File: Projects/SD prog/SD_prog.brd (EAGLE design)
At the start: 11 x 24.6 mm, 6 parts

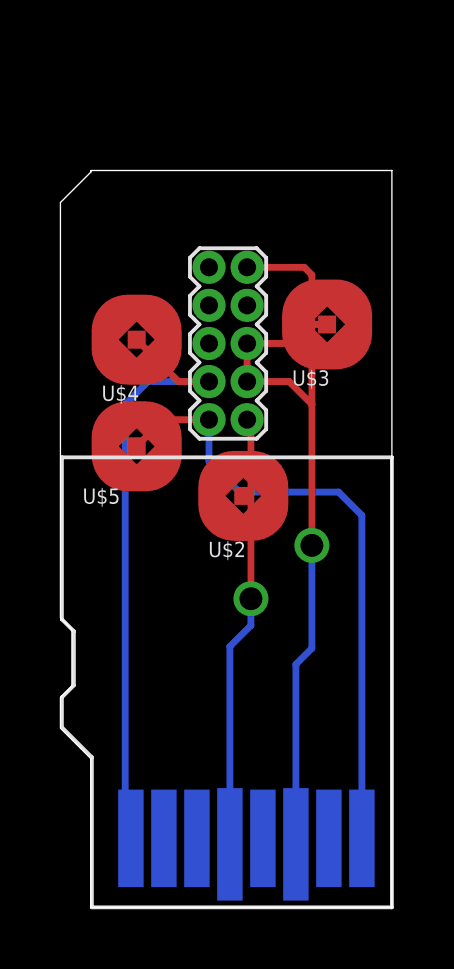
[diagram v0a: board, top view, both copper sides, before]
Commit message: Order @ Boktech
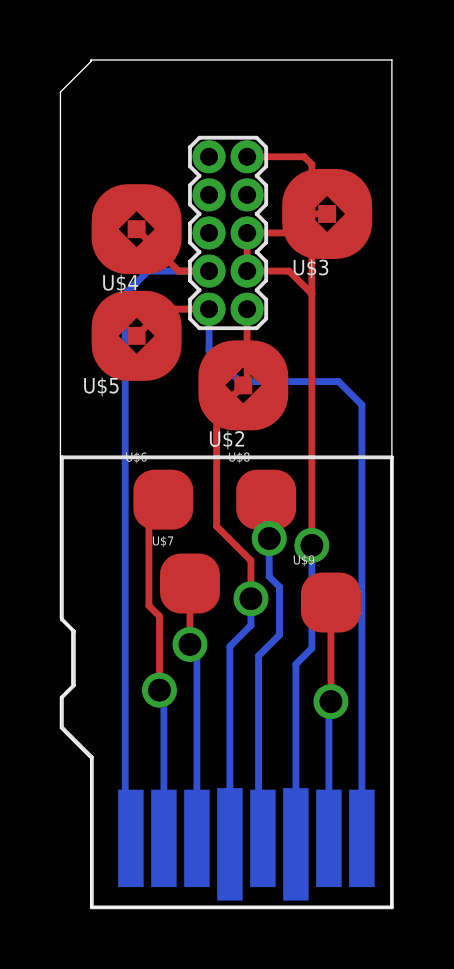
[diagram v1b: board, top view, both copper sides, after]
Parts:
- added U$6, U$7, U$8, U$9: TESTPOINT_22, test_points:TESTPOINT_22
- moved U$4 3.68 mm to (1.52, 22.6)
- moved U$2 3.68 mm to (5.08, 17.4)
- moved U$1 3.68 mm to (4.57, 22.5)
- moved U$3 3.68 mm to (7.87, 23.1)
- moved U$5 3.68 mm to (1.52, 19.1)
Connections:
- new net N$1: B1.CD/DAT3, U$6.P$1
- new net N$2: B1.CMD, U$7.P$1
- new net N$3: B1.CLK, U$8.P$1
- new net N$4: B1.DAT0, U$9.P$1
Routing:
- net N$3: track 0.00 -> 11.8 mm, vias 0 -> 1
- net N$1: track 0.00 -> 11.7 mm, vias 0 -> 1
- net N$2: track 0.00 -> 8.59 mm, vias 0 -> 1
- net N$4: track 0.00 -> 7.89 mm, vias 0 -> 1
- net VCC: track 14.5 -> 19.2 mm
- net SWDCLK/TCK: track 20.6 -> 24.3 mm
- net SWDIO/TMS: track 20.8 -> 24.5 mm
- net GND: track 28.1 -> 31.8 mm
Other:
- board size 11 x 24.6 mm -> 11 x 28.2 mm
